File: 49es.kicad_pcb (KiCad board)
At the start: 2 copper layers, 94 x 72.4 mm, 33 parts, among them J1 Conn_02x13_Row_Letter_Last, Q1 Q_PNP_BCE, Q2 Q_PNP_BCE, Q3 Q_PNP_BCE, Q4 Q_PNP_BCE, Q5 Q_PNP_BCE, Q6 Q_PNP_BCE, Q7 Q_PNP_BCE

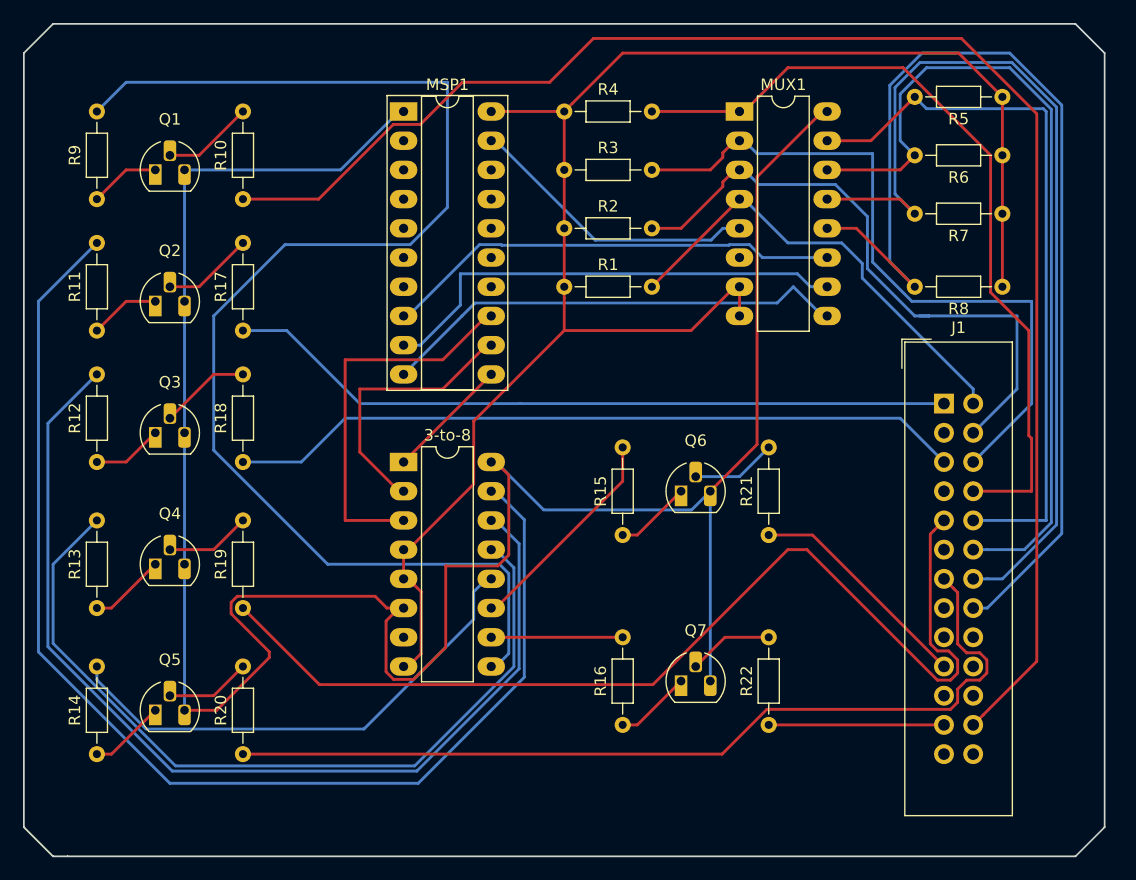
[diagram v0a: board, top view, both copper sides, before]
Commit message: fixes
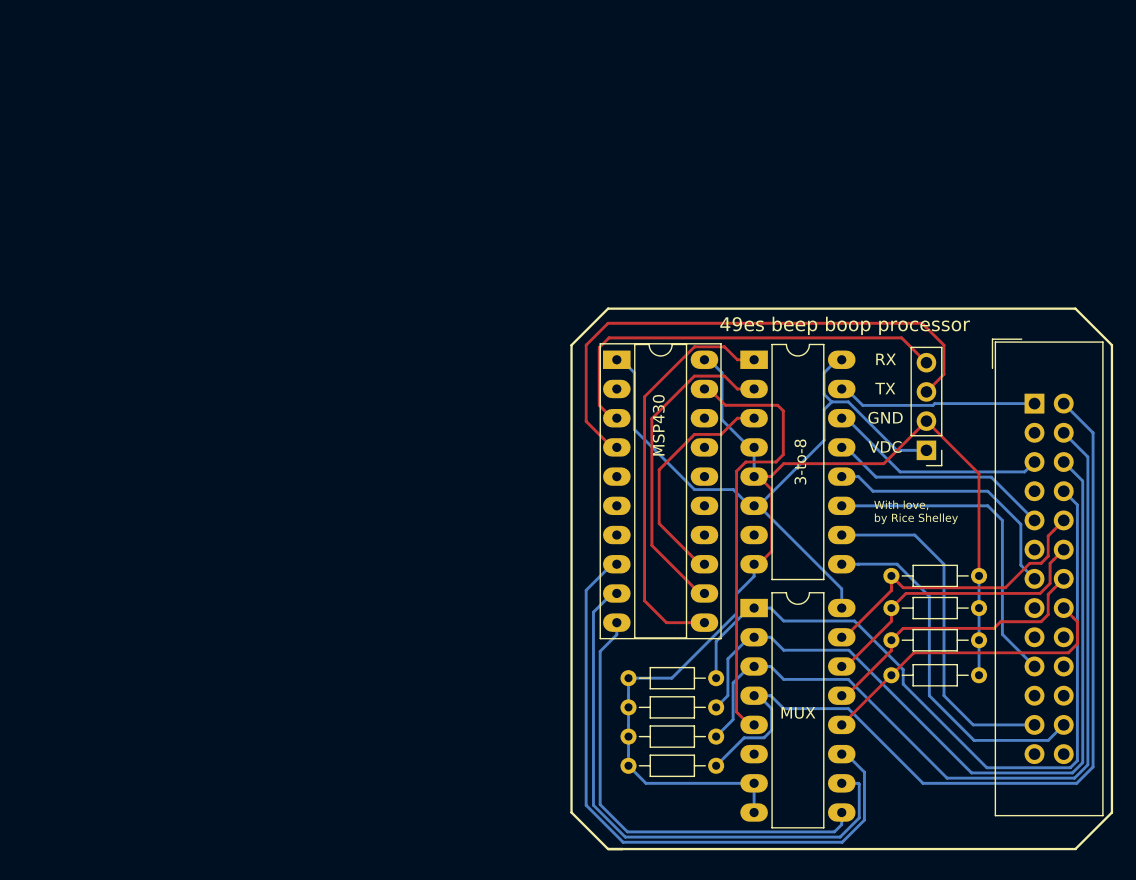
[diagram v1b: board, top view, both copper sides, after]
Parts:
- removed MSP1: MSP430G2553IN20, Package_DIP:DIP-20_W7.62mm_Socket_LongPads
- removed MUX1: 74LS251, Package_DIP:DIP-16_W7.62mm_LongPads
- removed Q1, Q2, Q3, Q4, Q5, Q6, Q7: Q_PNP_BCE, Package_TO_SOT_THT:TO-92_HandSolder
- removed R10, R11, R12, R13, R14, R15, R16, R17, R18, R19, R20, R21, R22, R9: R_US, Resistor_THT:R_Axial_DIN0204_L3.6mm_D1.6mm_P7.62mm_Horizontal
- added J2: Conn_01x04, Connector_PinHeader_2.54mm:PinHeader_1x04_P2.54mm_Vertical, F.Cu at (185.2, 70.1)
- added MSP430: MSP430G2553IN20, Package_DIP:DIP-20_W7.62mm_Socket_LongPads, F.Cu at (158.2, 62.2)
- added MUX: 74LS251, Package_DIP:DIP-16_W7.62mm_LongPads, F.Cu at (170.2, 83.8)
- moved R4 49.6 mm to (159.3, 89.9)
- moved R3 47.1 mm to (159.3, 92.5)
- moved R2 44.5 mm to (159.3, 95.0)
- moved R1 42.0 mm to (159.3, 97.5)
- moved R5 41.7 mm to (189.7, 81.0)
- moved R6 39.4 mm to (189.7, 83.8)
- moved R7 37.1 mm to (189.7, 86.6)
- moved R8 33.8 mm to (189.7, 89.7)
- moved 3-to-8 31.8 mm to (170.2, 62.2)
- moved J1 7.87 mm to (194.6, 66.0)
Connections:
- J1 pad 1: Net-(J1-Pad1) -> Net-(3-to-8-Pad15)
- J1 pad 13: Net-(J1-Pad13) -> Net-(3-to-8-Pad12)
- J1 pad 19: Net-(J1-Pad19) -> Net-(3-to-8-Pad11)
- J1 pad 23: Net-(J1-Pad23) -> Net-(3-to-8-Pad10)
- J1 pad 24: Net-(J1-Pad24) -> Net-(3-to-8-Pad9)
- J1 pad 5: Net-(J1-Pad5) -> Net-(3-to-8-Pad14)
- J1 pad 9: Net-(J1-Pad9) -> Net-(3-to-8-Pad13)
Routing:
- net +3V3: track 209.6 -> 58.8 mm
- net Net-(J1-Pad24): track 133.0 -> 0.00 mm
- net Net-(J1-Pad9): track 90.0 -> 0.00 mm
- net Net-(3-to-8-Pad15): track 106.1 -> 17.4 mm
- net Net-(3-to-8-Pad9): track 117.4 -> 31.3 mm
- net Net-(J1-Pad13): track 78.7 -> 0.00 mm
- net Net-(3-to-8-Pad14): track 88.7 -> 19.1 mm
- net Net-(J1-Pad16): track 93.8 -> 27.0 mm
- net Net-(J1-Pad5): track 64.1 -> 0.00 mm
- net Net-(J1-Pad1): track 63.6 -> 0.00 mm
- net Net-(J1-Pad14): track 81.9 -> 25.1 mm
- net Net-(3-to-8-Pad13): track 71.6 -> 19.4 mm
- net Net-(J1-Pad12): track 73.3 -> 25.2 mm
- net Net-(J2-Pad3): track 0.00 -> 47.6 mm
- net GND: track 140.0 -> 101.1 mm
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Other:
- board outline removed
- rule pad_to_mask_clearance: 0.2 -> 0
- rule trace_min: 0.2 -> 0.25
- board text added: "49es beep boop processor"
- board text added: "GND"
- board text added: "RX"
- board text added: "TX"
- board text added: "VDC"
- board text added: "With love, by Rice Shelley"
